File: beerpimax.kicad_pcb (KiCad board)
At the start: 2 copper layers, 4 parts, among them J1 Raspberry_Pi_2_3, J2 SSR Terminal, U1 MAX31865, U2 MAX31865

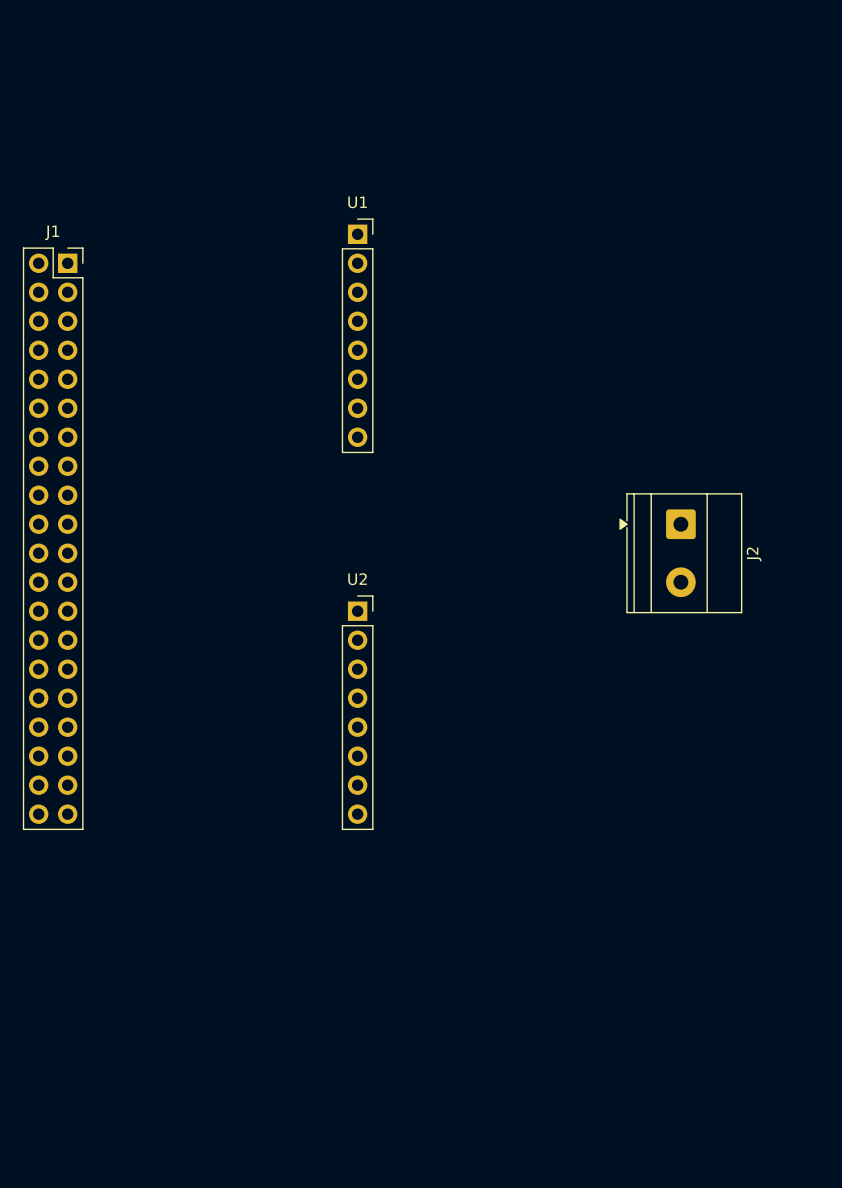
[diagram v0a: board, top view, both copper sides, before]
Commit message: board layout done
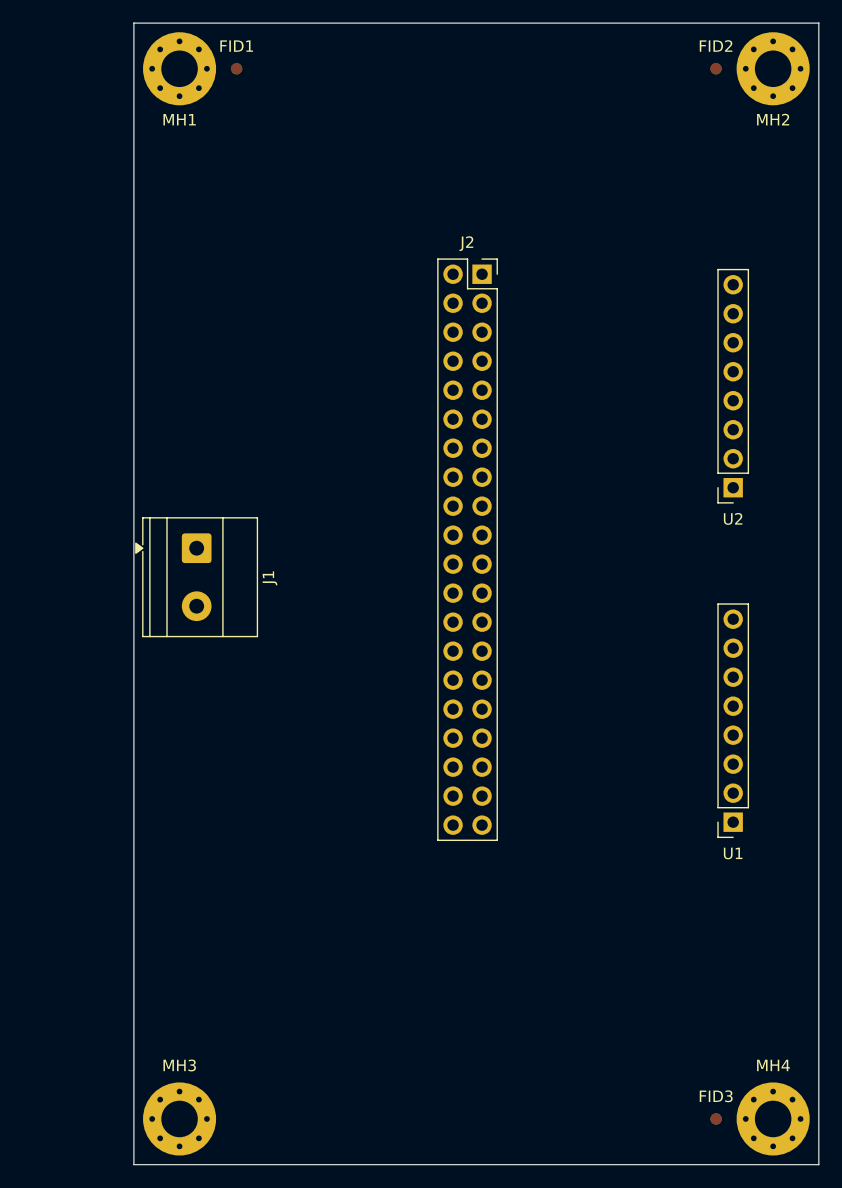
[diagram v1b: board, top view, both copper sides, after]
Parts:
- added FID1: Fiducial, Fiducial:Fiducial_1mm_Mask2mm, F.Cu at (154.5, 49.0)
- added FID2: Fiducial, Fiducial:Fiducial_1mm_Mask2mm, F.Cu at (196.5, 49.0)
- added FID3: Fiducial, Fiducial:Fiducial_1mm_Mask2mm, F.Cu at (196.5, 141.0)
- added MH1: M3, MountingHole:MountingHole_3.2mm_M3_Pad_Via, F.Cu at (149.5, 49.0)
- added MH2: M3, MountingHole:MountingHole_3.2mm_M3_Pad_Via, F.Cu at (201.5, 49.0)
- added MH3: M3, MountingHole:MountingHole_3.2mm_M3_Pad_Via, F.Cu at (149.5, 141.0)
- added MH4: M3, MountingHole:MountingHole_3.2mm_M3_Pad_Via, F.Cu at (201.5, 141.0)
- J1: value Raspberry_Pi_2_3 -> SSR Terminal; footprint Connector_PinSocket_2.54mm:PinSocket_2x20_P2.54mm_Vertical -> TerminalBlock_Phoenix:TerminalBlock_Phoenix_MKDS-1,5-2-5.08_1x02_P5.08mm_Horizontal
- J2: value SSR Terminal -> Raspberry_Pi_2_3; footprint TerminalBlock_Phoenix:TerminalBlock_Phoenix_MKDS-1,5-2-5.08_1x02_P5.08mm_Horizontal -> Connector_PinSocket_2.54mm:PinSocket_2x20_P2.54mm_Vertical
- moved U1 61.1 mm to (198.0, 115.0), turned to 180 degrees
- moved U2 34.6 mm to (198.0, 85.7), turned to 180 degrees
- moved J2 28.0 mm to (176.0, 67.0), turned to 0 degrees
- moved J1 27.4 mm to (151.0, 91.0), turned to -90 degrees
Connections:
- J1 pad 1: +3V3 -> /SSRGPIO18
- J1 pad 2: unconnected-(J1-5V-Pad2) -> GND
- J2 pad 1: Net-(J1-GPIO18/PWM0) -> +3V3
- J2 pad 2: GND -> unconnected-(J2-5V-Pad2)_1
- U1 pad 4: /SCLK -> /SPISCLK
- U1 pad 5: /MISO -> /SPIMISO
- U1 pad 6: /MOSI -> /SPIMOSI
- U1 pad 7: /GPIO7 -> /SPIGPIO7
- U2 pad 4: /SCLK -> /SPISCLK
- U2 pad 5: /MISO -> /SPIMISO
- U2 pad 6: /MOSI -> /SPIMOSI
- U2 pad 7: /GPIO8 -> /SPIGPIO8
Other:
- board outline added: 60 x 100 mm
- rule pad_to_mask_clearance: 0 -> 0.1
